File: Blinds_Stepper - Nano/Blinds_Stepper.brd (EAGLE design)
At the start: 69.5 x 67.3 mm, 22 parts

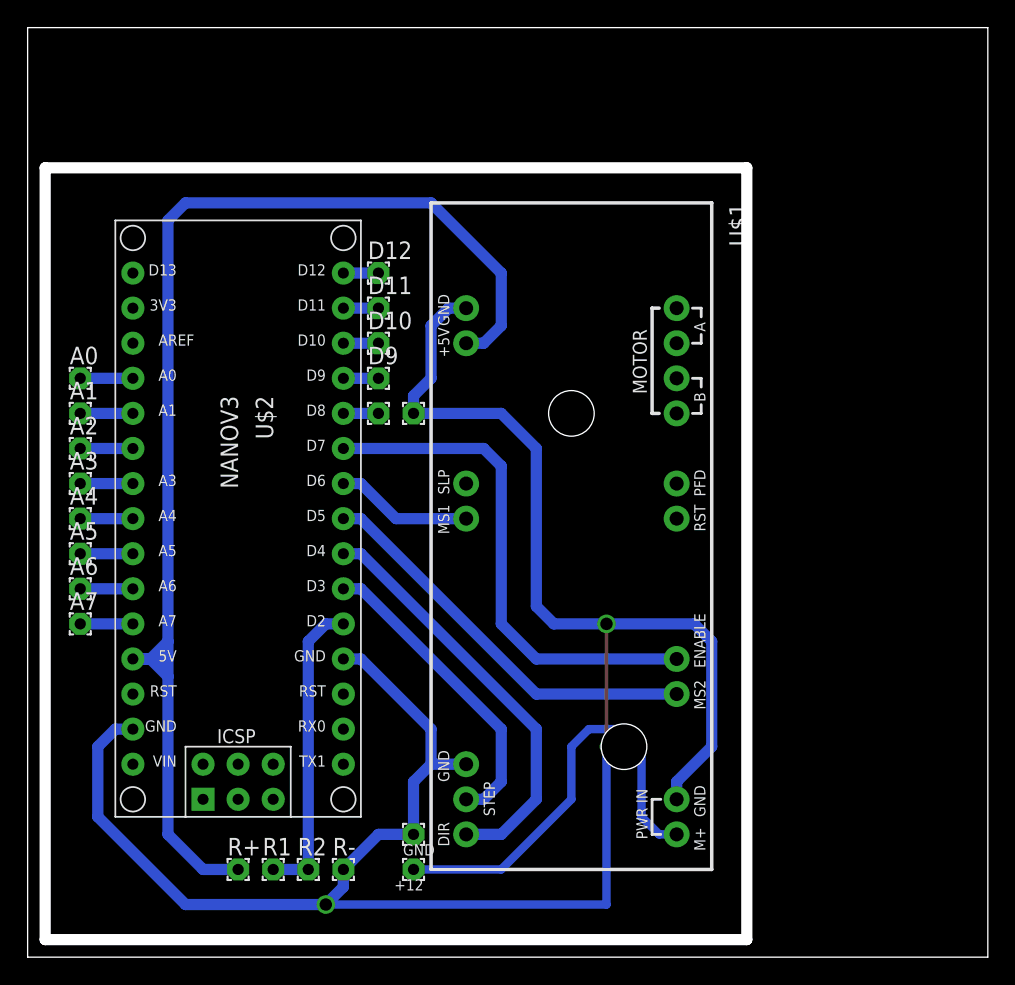
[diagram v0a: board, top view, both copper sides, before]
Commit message: clean up Blinds Stepper
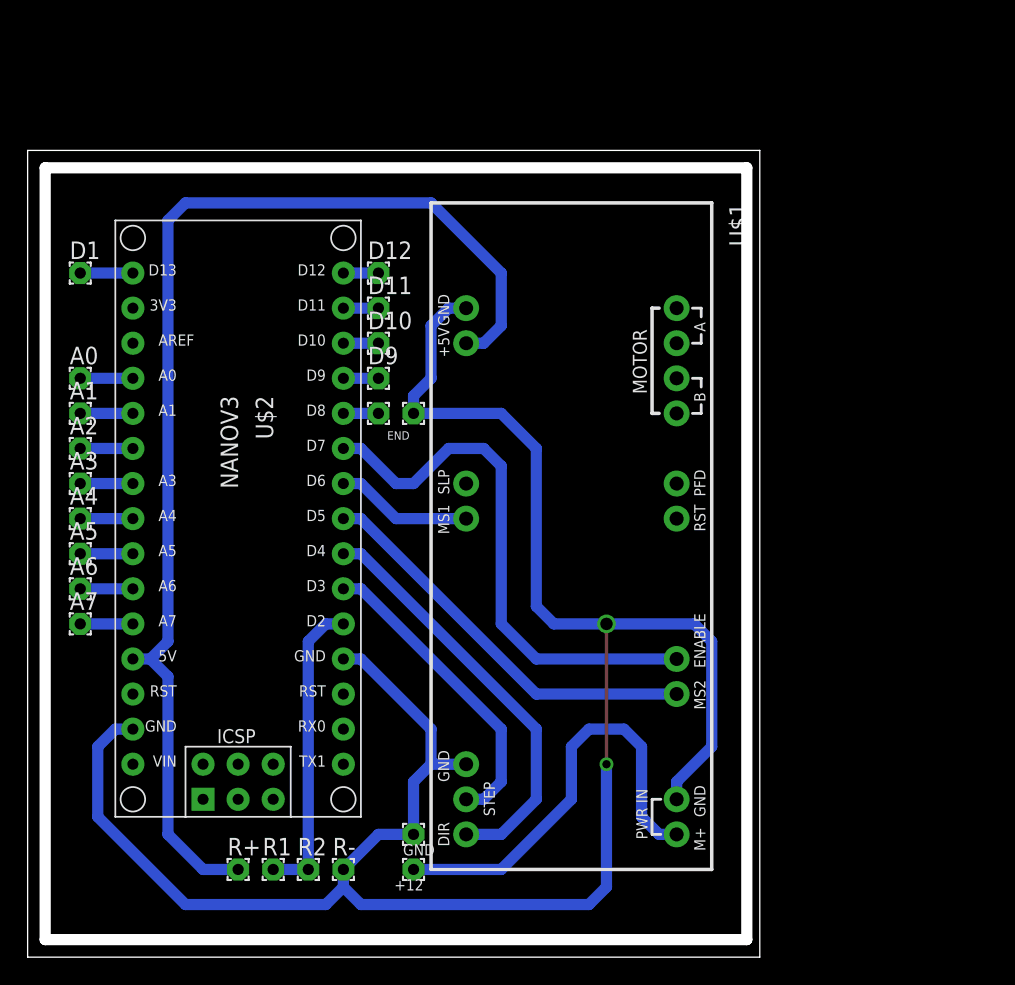
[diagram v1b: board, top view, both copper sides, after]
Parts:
- added D1: (no value), wirepad:1,6/0,8
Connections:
- new net D13: D1.1, U$2.D13
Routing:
- net 5V: track 91.6 -> 86.5 mm
- net D13: track 0.00 -> 3.81 mm
- net ENBL: track 37.1 -> 39.2 mm
- net GND: track 153.8 -> 152.3 mm, vias 3 -> 2
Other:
- board size 69.5 x 67.3 mm -> 53 x 58.4 mm
- board text added: "END"
